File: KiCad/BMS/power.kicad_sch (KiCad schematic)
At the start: 14 parts, among them U3 ST1S14PHR, U4 LDL1117S33R

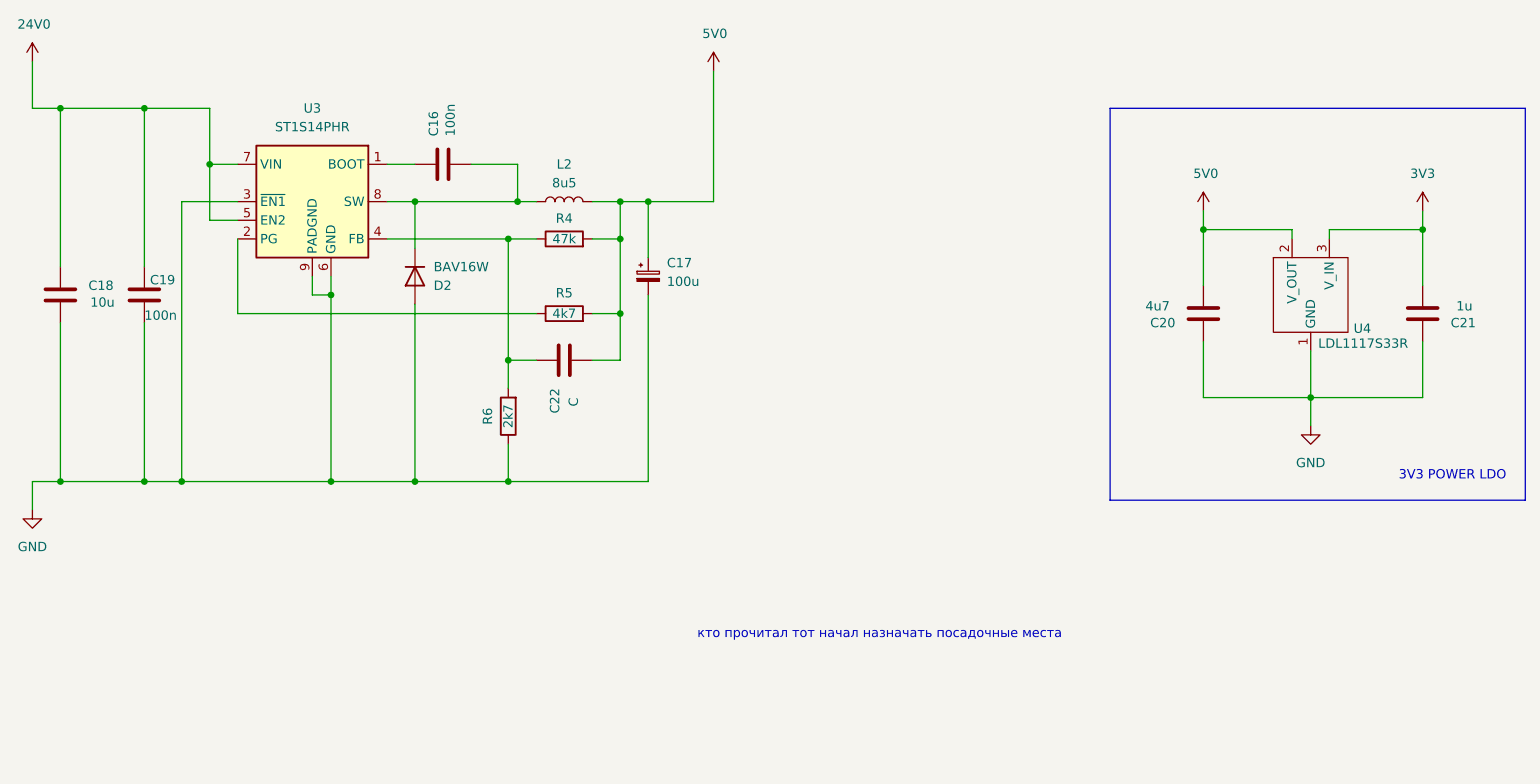
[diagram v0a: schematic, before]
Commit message: 22.03.2025
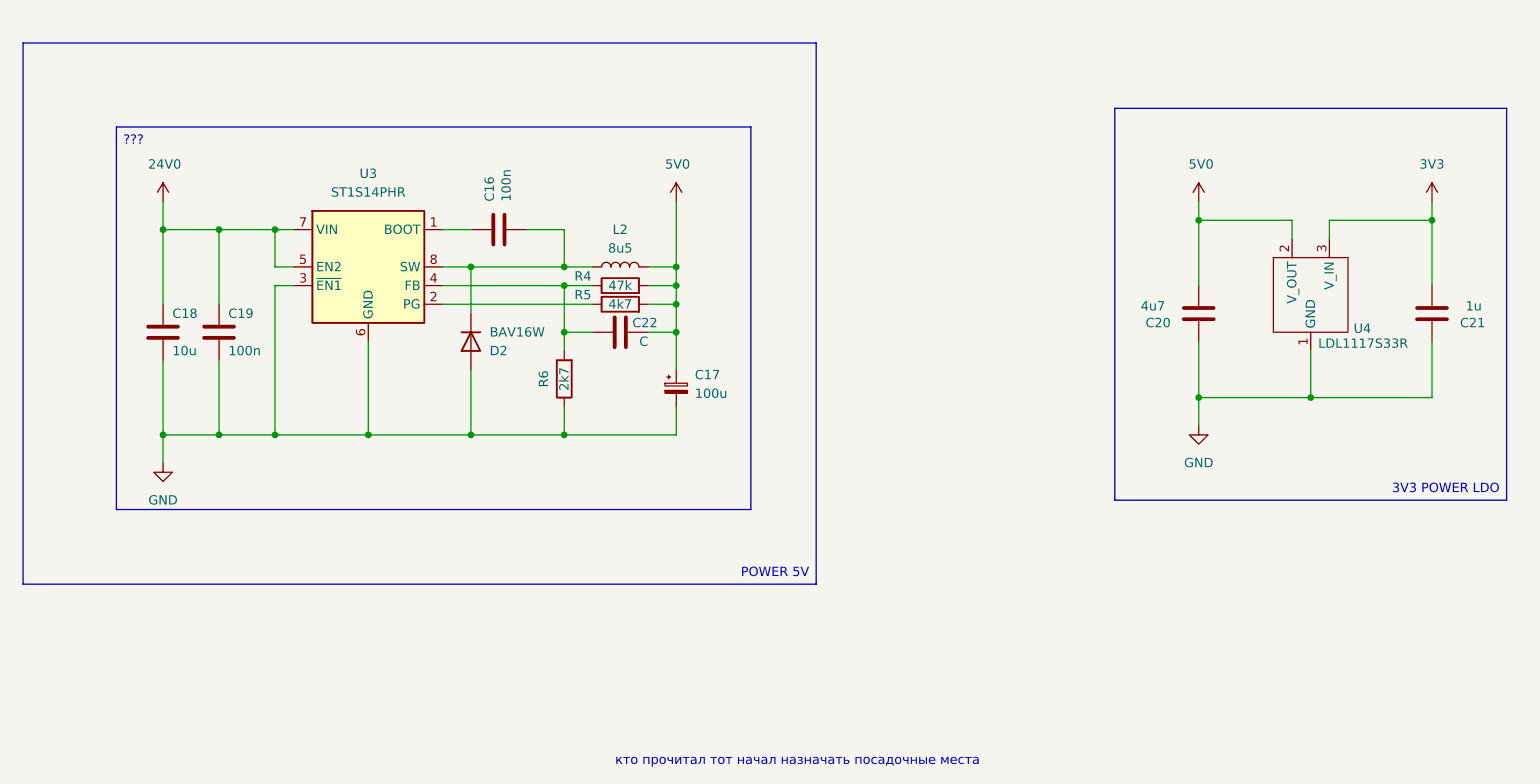
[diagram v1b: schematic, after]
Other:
- note removed: "3V3 POWER LDO"
- moved on the sheet: C16, C17, C18, C19, C20, C21, C22, D2, L2, R4, R5, R6
